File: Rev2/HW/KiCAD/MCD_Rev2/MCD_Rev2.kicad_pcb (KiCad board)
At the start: 2 copper layers, 196.3 x 114.7 mm, 76 parts, among them J1 DBUS_LOW, J2 DBUS_HIGH, J3 ABUS, J4 POWER, J5 JTAG, J6 Conn_01x02_Male, J7 DUART A, J8 DUART B, SW1 SW_Push, U1 XC9572XL-PC44, U10 STM1001LWX6F, U2 AS6C1008-55PCN, U3 AS6C1008-55PCN, U4 SST39SF020A-70-4C-PHE, U5 SST39SF020A-70-4C-PHE, U6 XR68C681CJ-F, U7 AP2114HA-3.3TRG1, U8 MAX6816EUS_T, U9 MC68000FN, Y1 ECS-100AX-036, Y2 ECS-100AX-080

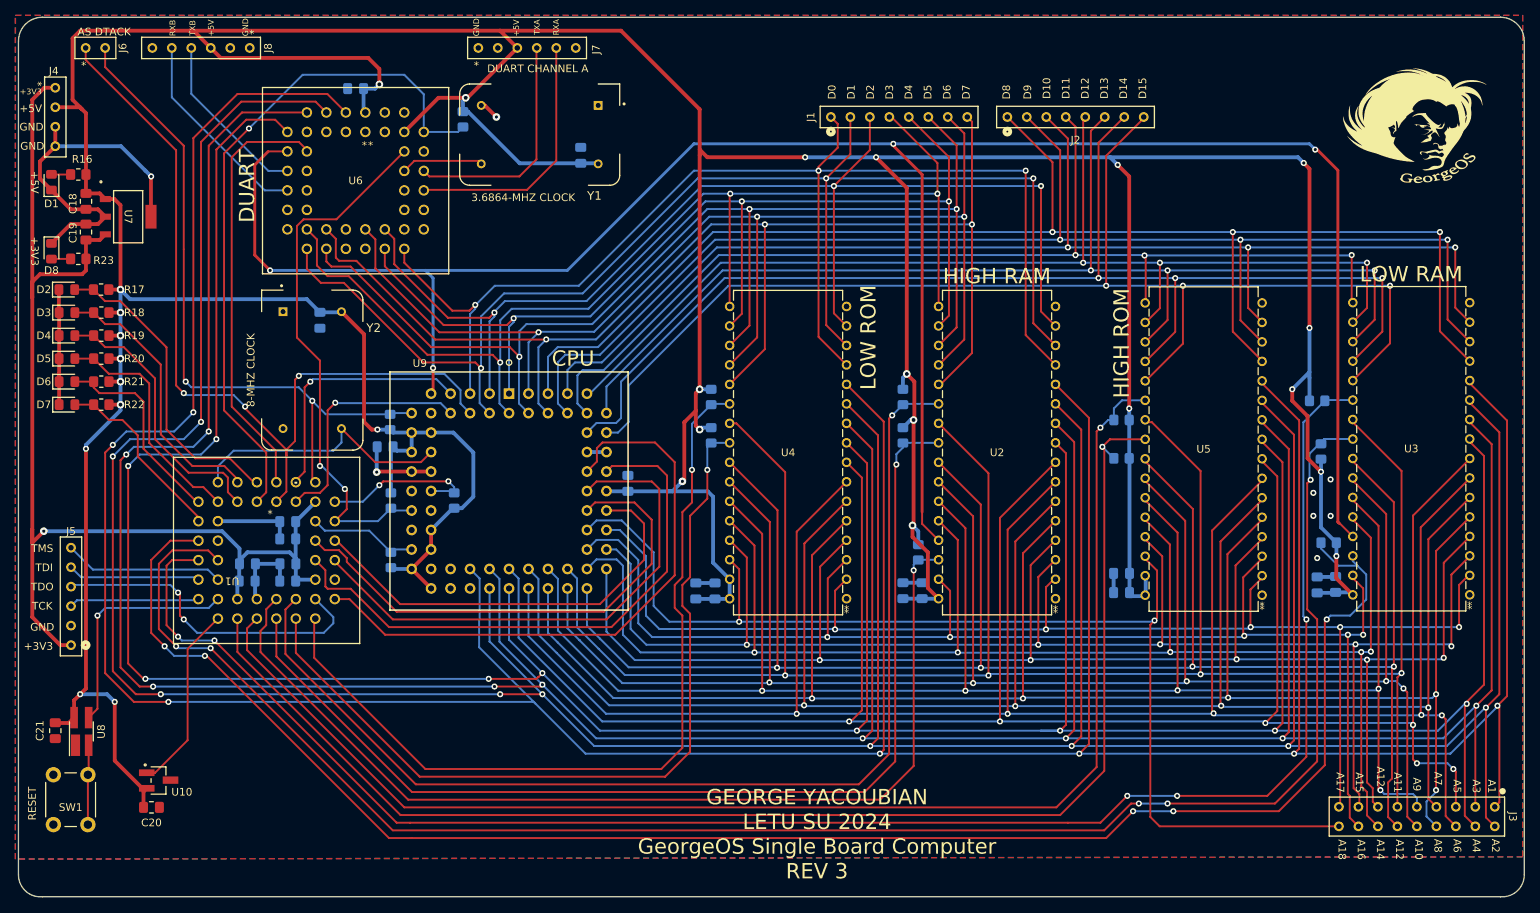
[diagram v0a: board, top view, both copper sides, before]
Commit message: filled in POURS
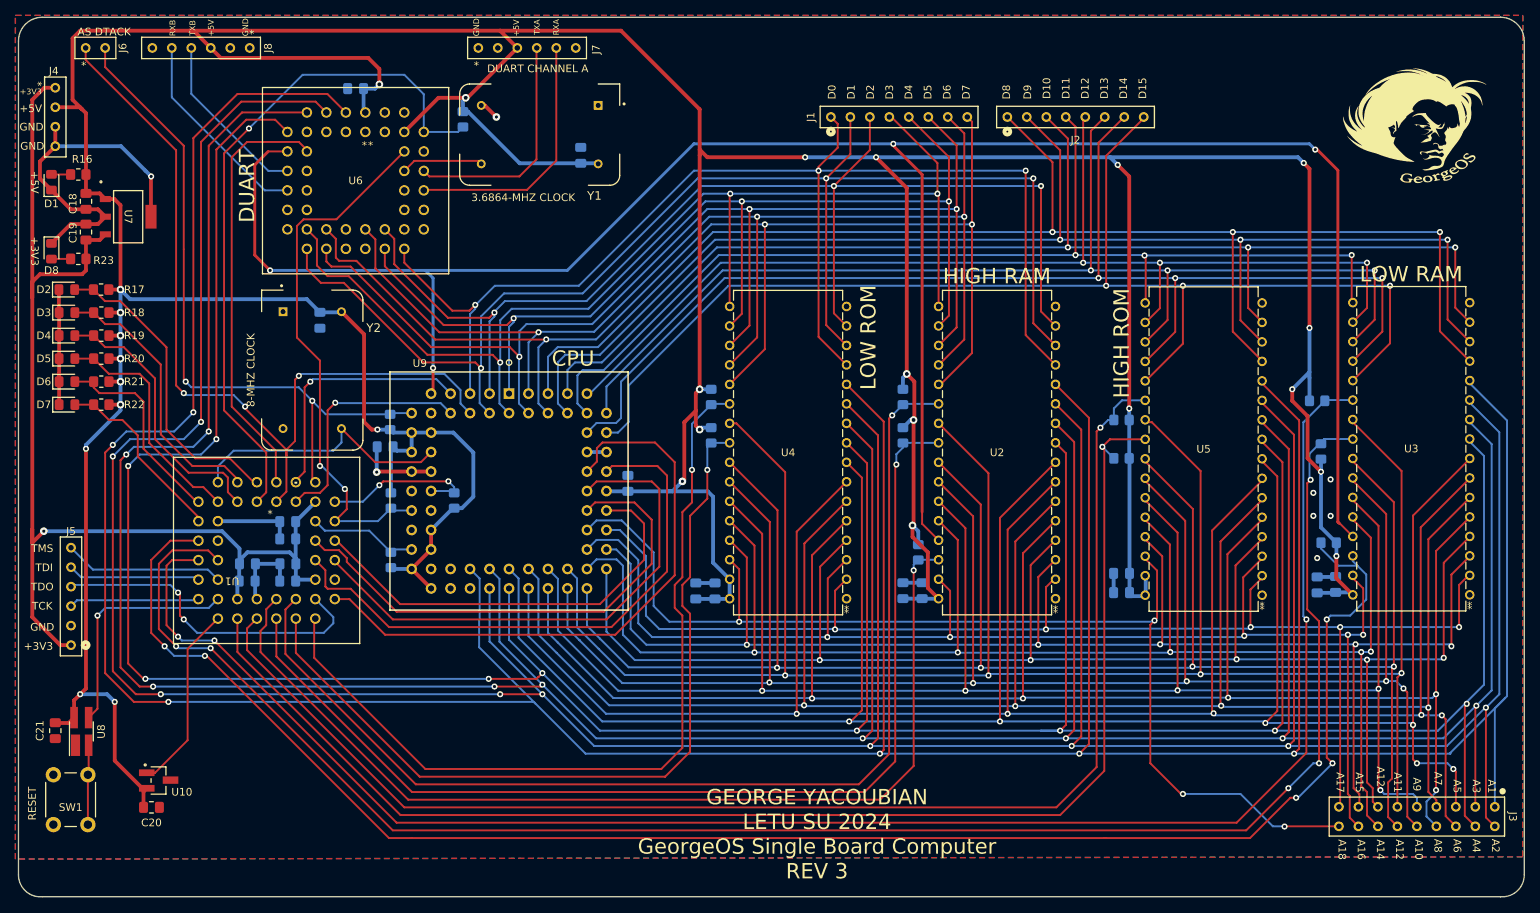
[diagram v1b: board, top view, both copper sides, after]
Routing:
- net A18: track 152.5 -> 148.5 mm, vias 2 -> 4
- net RAMHCE2: track 222.9 -> 224.2 mm
- net A1: track 521.2 -> 522.4 mm, vias 7 -> 6
- net RAMHOE: track 230.4 -> 230.9 mm
- net RAMHCE: track 226.5 -> 226.2 mm, vias 5 -> 3
